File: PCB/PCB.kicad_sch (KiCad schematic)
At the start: 20 parts, among them SW1 SW4_Push, SW10 SW2_Push, SW11 SW3_Push, SW2 SW5_Push, SW3 RotaryEncoder_Switch, SW4 RotaryEncoder_Switch, SW5 SW6_Push, SW6 SW7_Push, SW7 SW_Push-Mode0, SW8 SW_Push-Mode1, SW9 SW1_Push, U4 ER_OLEDM0.91_1x-I2C, U5 MOUDLE-SEEEDUINO-XIAO

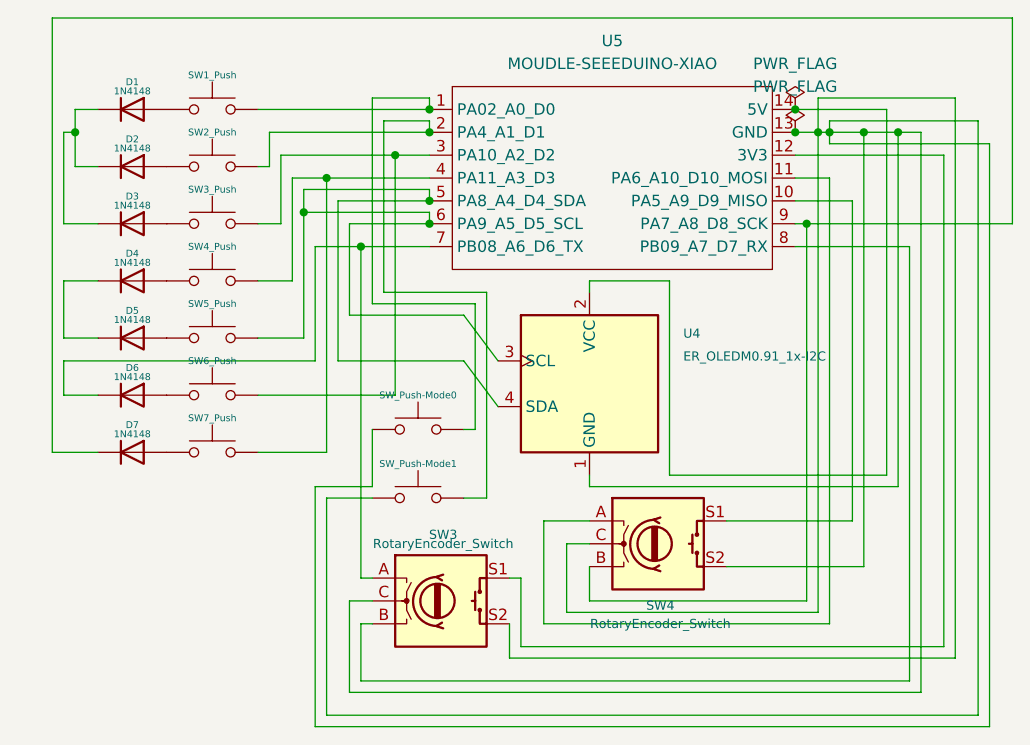
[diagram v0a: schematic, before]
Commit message: Add Hakin Pad bill of materials
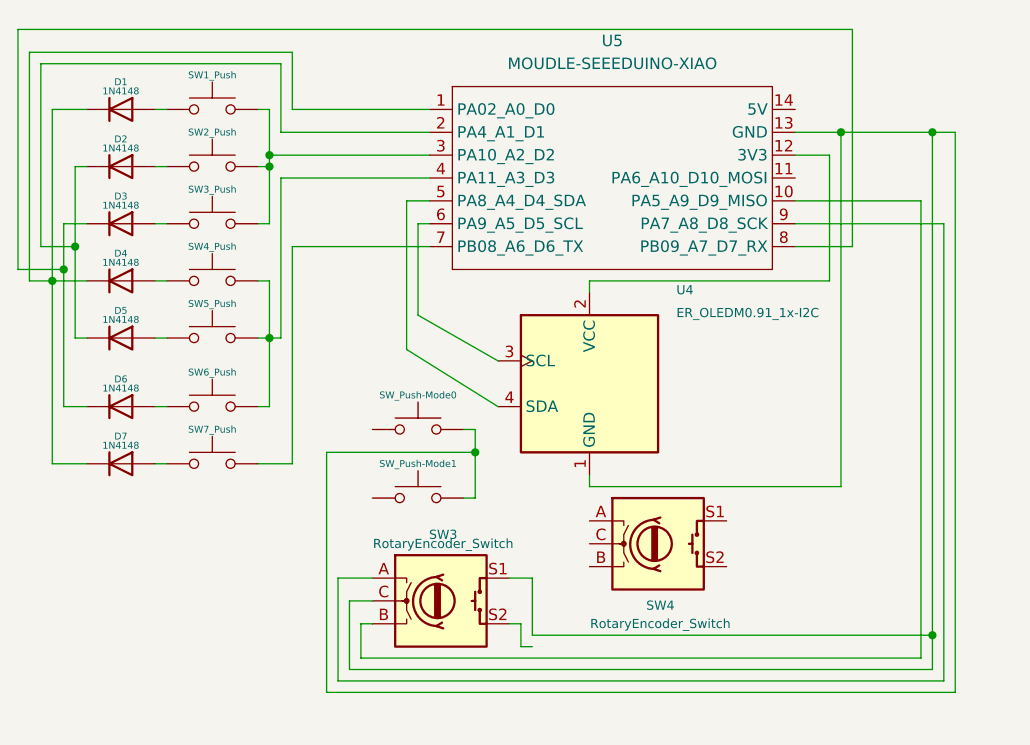
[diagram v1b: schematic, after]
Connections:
- net at SW11.2, U5.3 (PA10_A2_D2): now also SW10.2, SW9.2; no longer SW5.2
- net at SW1.2, U5.4 (PA11_A3_D3): now also SW2.2, SW5.2; no longer SW6.2
- net at U5.10 (PA5_A9_D9_MISO): now also SW3.B; no longer SW4.S1
- net at U5.11 (PA6_A10_D10_MOSI): no longer SW4.A
- net at U5.12 (3V3): now also U4.2 (VCC); no longer SW3.S1
- net at U5.14 (5V): no longer U4.2 (VCC)
- net at U5.8 (PB09_A7_D7_RX): now also D3.1 (K), D6.1 (K); no longer SW3.B
- net at D5.1 (K): now also D2.1 (K), U5.2 (PA4_A1_D1); no longer D4.1 (K)
- new net: SW6.2, U5.7 (PB08_A6_D6_TX)
- new net: D1.1 (K), D4.1 (K), D7.1 (K), U5.1 (PA02_A0_D0)
- new net: SW3.C, SW3.S1, SW7.2, SW8.2, U4.1 (GND), U5.13 (GND)
- new net: U4.4 (SDA), U5.5 (PA8_A4_D4_SDA)
- new net: U4.3 (SCL), U5.6 (PA9_A5_D5_SCL)
- new net: SW3.A, U5.9 (PA7_A8_D8_SCK)
- now unconnected: SW3.S2, SW4.B, SW4.C, SW4.S2, SW7.1, SW8.1
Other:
- moved on the sheet: D1, D2, D3, D4, D5, D6, D7
